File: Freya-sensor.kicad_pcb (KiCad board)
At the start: 2 copper layers, 50 x 15 mm, 24 parts, among them J1 Grove, J2 wires, Q1 BS170, Q2 BS170, U1 BME680, U2 VEML6030, U3 MIC5225-3.3YM5, U4 AS7331

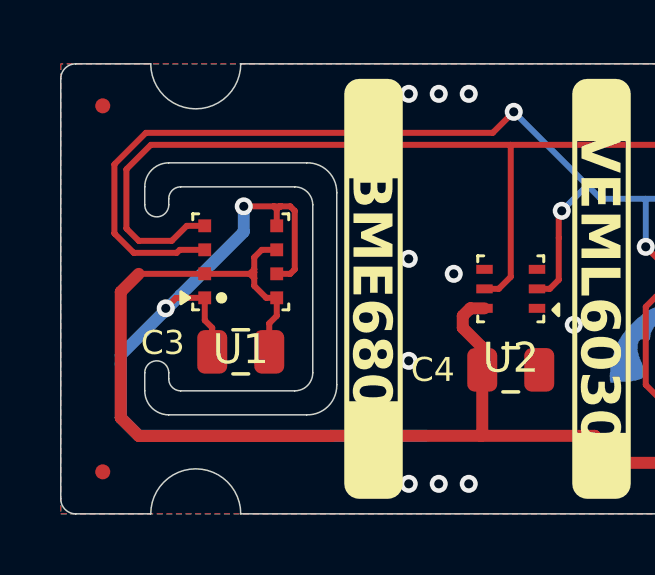
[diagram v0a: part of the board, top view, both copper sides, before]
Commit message: Update documentation
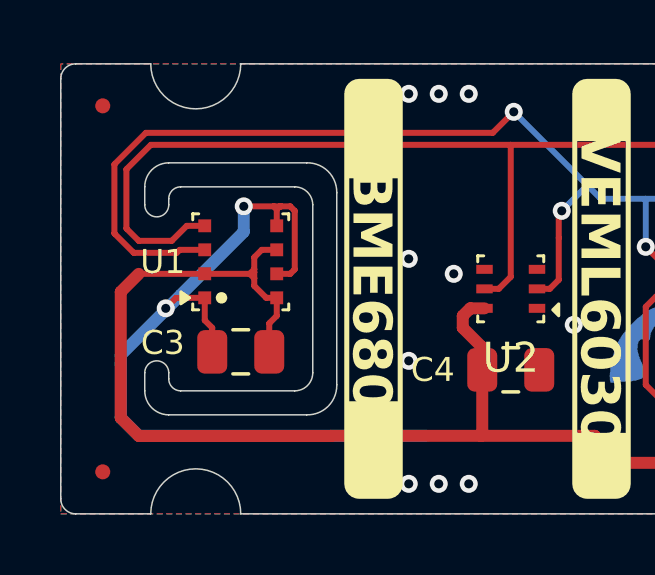
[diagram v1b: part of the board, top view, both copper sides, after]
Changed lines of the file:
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@@
 		(descr "Bosch BME680 temperature/humidity/pressure/gas sensor")
 		(property "Reference" "U1"
-			(at -2.915 0 180)
+			(at 0 -2.6 180)
 			(layer "F.SilkS")
 			(effects
 				(font
-					(size 1 1)
+					(size 0.8 0.8)
 					(thickness 0.15)
 				)
